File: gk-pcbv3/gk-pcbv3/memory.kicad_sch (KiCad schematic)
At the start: 25 parts, among them J4 Micro_SD_Card_Det2, U17 S80KS5122GABHI020, U5 S26KS128SDPBHI020, U6 S80KS5122GABHI020, U8 TPS2041BDBV

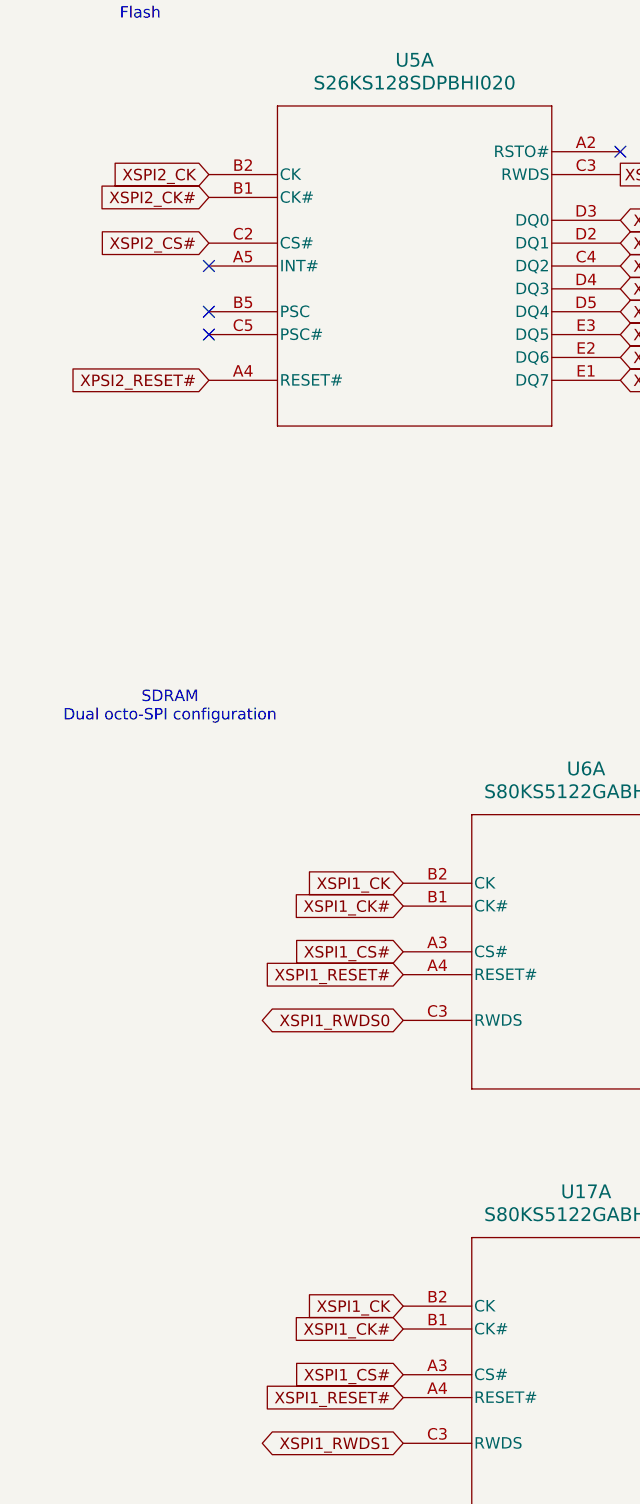
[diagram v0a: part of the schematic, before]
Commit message: hardware changes
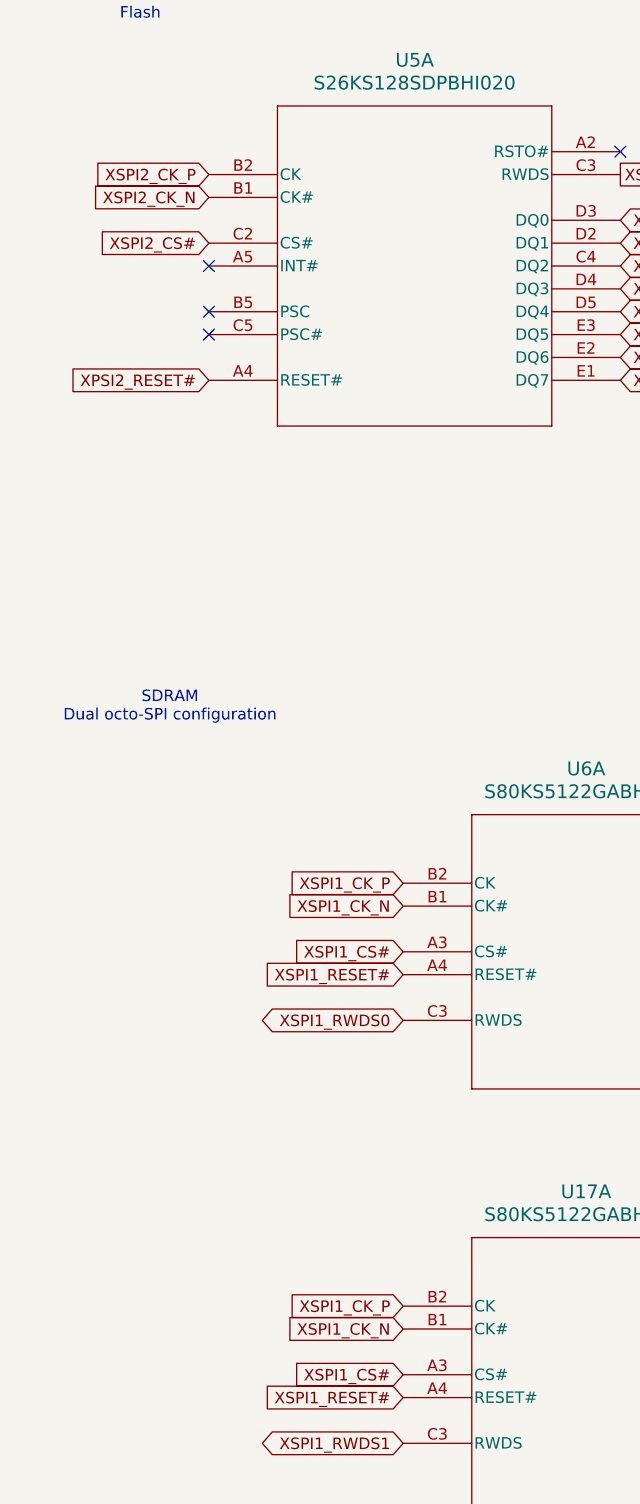
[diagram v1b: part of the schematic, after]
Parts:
- U17, U6: footprint STM32H7S7:PG-BGA-24-801 -> STM32H7S7:BGA24_Hyperbus
- U5: footprint STM32H7S7:BGA24_S26KS512SDPBHI020_CYP_INF -> STM32H7S7:BGA24_Hyperbus
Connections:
- net XSPI1_CK renamed XSPI1_CK_P
- net XSPI1_CK# renamed XSPI1_CK_N
- net XSPI2_CK renamed XSPI2_CK_P
- net XSPI2_CK# renamed XSPI2_CK_N
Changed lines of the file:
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@@
 		)
 	)
-	(global_label "XSPI1_CK"
+	(global_label "XSPI1_CK_P"
 		(shape input)
 		(at 53.34 116.84 180)
@@
 		)
 	)
-	(global_label "XSPI1_CK#"
+	(global_label "XSPI1_CK_N"
 		(shape input)
 		(at 53.34 166.37 180)
@@
 		)
 	)
-	(global_label "XSPI2_CK#"
+	(global_label "XSPI2_CK_N"
 		(shape input)
 		(at 31.75 40.64 180)
@@
 		)
 	)
-	(global_label "XSPI1_CK#"
+	(global_label "XSPI1_CK_N"
 		(shape input)
 		(at 53.34 119.38 180)
@@
 		)
 	)
-	(global_label "XSPI1_CK"
+	(global_label "XSPI1_CK_P"
 		(shape input)
 		(at 53.34 163.83 180)
@@
 		)
 	)
-	(global_label "XSPI2_CK"
+	(global_label "XSPI2_CK_P"
 		(shape input)
 		(at 31.75 38.1 180)
@@
 			)
 		)
-		(property "Footprint" "STM32H7S7:PG-BGA-24-801"
+		(property "Footprint" "STM32H7S7:BGA24_Hyperbus"
 			(at 53.34 163.83 0)
 			(effects
@@
 			)
 		)
-		(property "Footprint" "STM32H7S7:BGA24_S26KS512SDPBHI020_CYP_INF"
+		(property "Footprint" "STM32H7S7:BGA24_Hyperbus"
 			(at 102.87 36.83 0)
 			(effects
@@
 			)
 		)
-		(property "Footprint" "STM32H7S7:PG-BGA-24-801"
+		(property "Footprint" "STM32H7S7:BGA24_Hyperbus"
 			(at 166.37 120.65 0)
 			(effects
@@
 			)
 		)
-		(property "Footprint" "STM32H7S7:BGA24_S26KS512SDPBHI020_CYP_INF"
+		(property "Footprint" "STM32H7S7:BGA24_Hyperbus"
 			(at 31.75 38.1 0)
 			(effects
@@
 			)
 		)
-		(property "Footprint" "STM32H7S7:PG-BGA-24-801"
+		(property "Footprint" "STM32H7S7:BGA24_Hyperbus"
 			(at 156.21 120.65 0)
 			(effects
@@
 			)
 		)
-		(property "Footprint" "STM32H7S7:PG-BGA-24-801"
+		(property "Footprint" "STM32H7S7:BGA24_Hyperbus"
 			(at 53.34 116.84 0)
 			(effects
